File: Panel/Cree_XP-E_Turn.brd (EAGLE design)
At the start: 50 x 50 mm, 10 parts

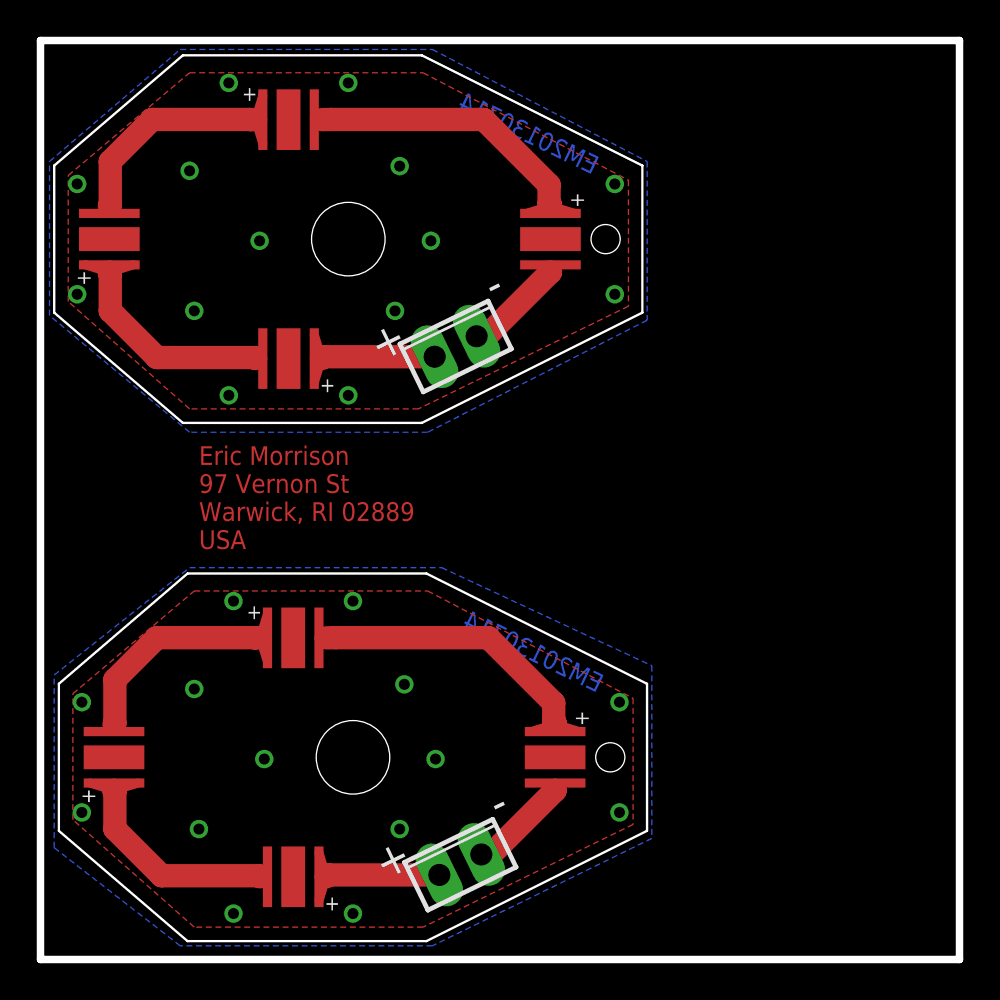
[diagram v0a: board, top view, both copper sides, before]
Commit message: Turn and Tail combined Panel
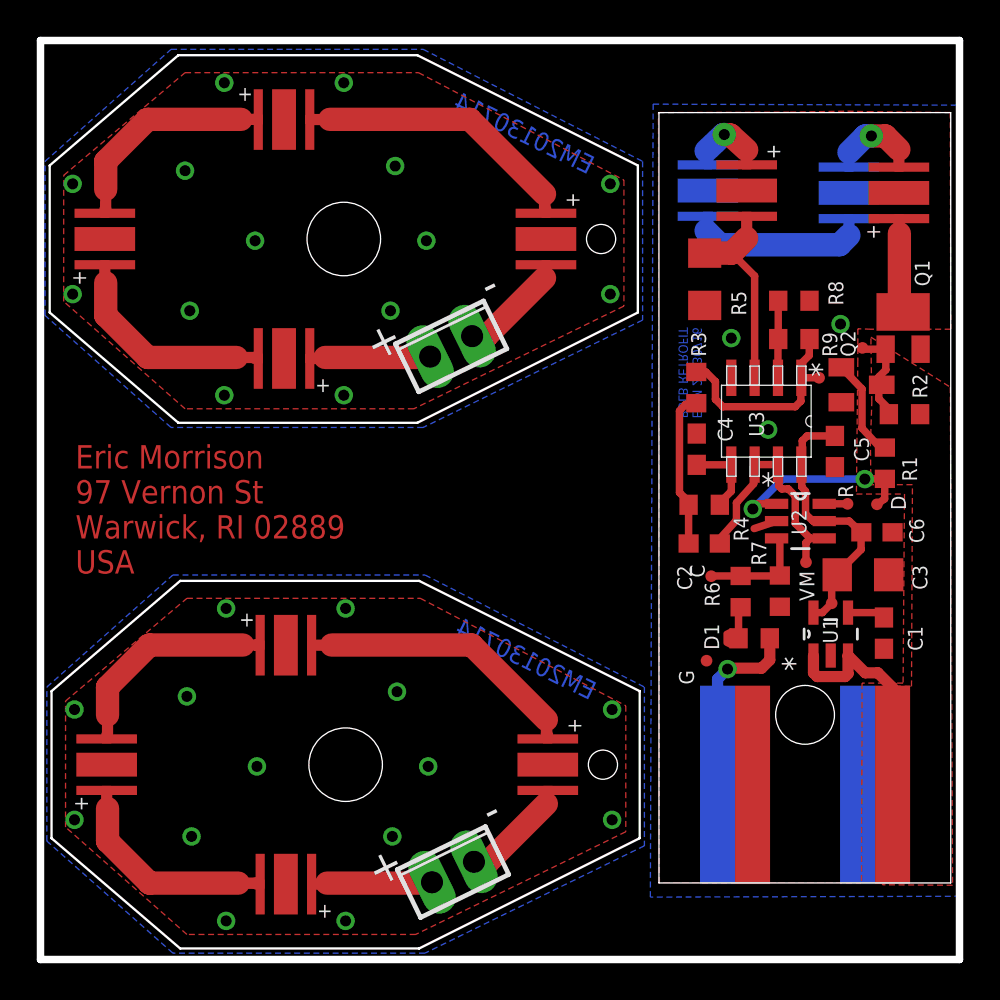
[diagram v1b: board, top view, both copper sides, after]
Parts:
- added +5V, GND, MEASURE, OUTA, PWM, RESET, TPICLK, TPIDATA: TPI, Personal:TPI_PAD
- added C1: 10n, resistor:C0603
- added C2, C4, C5, C6: .1u, resistor:C0603
- added C3: 47u, resistor:C1206
- added D1: DIODE_0603, Combined:D0603
- added DRILEGEND: (no value), drilegend:DRILEGEND
- added LED10, LED11, LED12, LED9: LUXEON_REBELCREE_XP-E, Combined:CREE_XP-E
- added Q1: SI2301CDS, Combined:SOT-23_POWER
- added Q2: BC846, transistor-neu-to92:SOT23
- added R1: 10k, resistor:R0603
- added R2, R7, R8: 1k, resistor:R0603
- added R3, R4: 3.9k, resistor:R0603
- added R5: .1, resistor:R1206
- added R6: 3.3k, resistor:R0603
- added R9: 28.7K, resistor:R0603
- added U$1: CON_TAILLIGHT, Combined:TAILLIGHT
- added U1: SPX5205M5-L-3-3, Exar_By_element14_Batch_1:SOT95P280X145-5N
- added U2: ATTINY5-TSHR, Atmel_By_element14_Batch_1:SOT95P280X145-6N
- added U3: MCP6L2-X_SN, Combined:SOIC8-N_MC
- moved LED3 0.57 mm to (2.60, 9.60)
- moved LED4 0.57 mm to (12.3, 3.10)
- moved LED1 0.57 mm to (26.6, 9.60)
- moved LED2 0.57 mm to (12.3, 16.1)
- moved X1 0.57 mm to (21.4, 3.76)
- moved X2 0.25 mm to (21.3, 32.4)
- moved LED6 0.25 mm to (12.2, 44.7)
- moved LED8 0.25 mm to (12.2, 31.7)
- moved LED7 0.25 mm to (2.50, 38.2)
- moved LED5 0.25 mm to (26.5, 38.2)
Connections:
- new net +14V: Q1.P$2, R2.1, U$1.H1, U1.1, U1.3
- new net BLINK: R6.1, R7.1, TPICLK.P$1, U2.3
- new net CROSSOVER: LED10.CT, LED11.AN
- new net D-: LED12.CT, R5.2, U3.3
- new net GND: C1.2, C3.2, C4.2, C5.2, C6.2, GND.P$1, LED10.TH, LED11.TH, LED12.TH, LED9.TH, Q2.2, R5.1, R7.2, R8.2, U$1.L1, U$1.L2, U1.2, U2.2, U3.4
- new net INA-: R8.1, R9.2, U3.2
- new net INB+: C4.1, R4.2, U3.5
- new net MEASURE: C2.1, MEASURE.P$1, U2.4, U3.6, U3.7
- new net MOSFET: R1.1, TPIDATA.P$1, U2.1
- new net N$10: C2.2, R3.2, R4.1
- new net N$11: D1.1A, U$1.H2
- new net N$12: D1.2C, R6.2
- new net N$13: LED11.CT, LED12.AN
- new net N$14: LED9.AN, Q1.P$3
- new net N$15: LED10.AN, LED9.CT
- new net N$7: C1.1, U1.4
- new net N$8: PWM.P$1, Q1.P$1, Q2.3, R2.2
- new net N$9: Q2.1, R1.2
- new net OUTA: OUTA.P$1, R3.1, R9.1, U3.1
- new net RESET: RESET.P$1, U2.6
- new net VCC: +5V.P$1, C3.1, C5.1, C6.1, U1.5, U2.5, U3.8
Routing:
- net VCC: track 0.00 -> 15.1 mm
- net MEASURE: track 0.00 -> 13.4 mm
- net D-: track 0.00 -> 12.4 mm
- net +14V: track 0.00 -> 12.4 mm
- net OUTA: track 0.00 -> 11.7 mm
- net MOSFET: track 0.00 -> 10.9 mm, vias 0 -> 2
- net N$11: track 0.00 -> 10.2 mm, vias 0 -> 1
- net CROSSOVER: track 0.00 -> 9.60 mm
- net N$10: track 0.00 -> 8.52 mm
- net BLINK: track 0.00 -> 6.13 mm
- net N$9: track 0.00 -> 5.47 mm
- net N$8: track 0.00 -> 5.36 mm
- net N$14: track 0.00 -> 4.97 mm
- net N$15: track 0.00 -> 4.76 mm, vias 0 -> 1
- net INB+: track 0.00 -> 4.38 mm
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- added copper zone on layer 1, net +14V
- added copper zone on layer 1, net GND
- added copper zone on layer 16, net GND
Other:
- outline, holes or cut-outs redrawn
- board text added: "C"
- board text added: "C1"
- board text added: "C2"
- board text added: "C3"
- board text added: "C4"
- board text added: "C5"
- board text added: "C6"
- board text added: "D"
- board text added: "D1"
- board text added: "EWM 20130716 BULB RETROFIT"
- board text added: "G"
- board text added: "M"
- board text added: "Q1"
- board text added: "Q2"
- board text added: "R"
- board text added: "R1"
- board text added: "R2"
- board text added: "R3"
- board text added: "R4"
- board text added: "R5"
- board text added: "R6"
- board text added: "R7"
- board text added: "R8"
- board text added: "R9"
- board text added: "U1"
- board text added: "U2"
- board text added: "U3"
- board text added: "V"
